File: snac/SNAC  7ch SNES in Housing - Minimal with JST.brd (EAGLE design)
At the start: 63.6 x 64.1 mm, 8 parts, among them U1 PMIC-LDO-XC6206P332MR-G(SOT23), X2 JST-XH-09-PIN-LONG-PAD

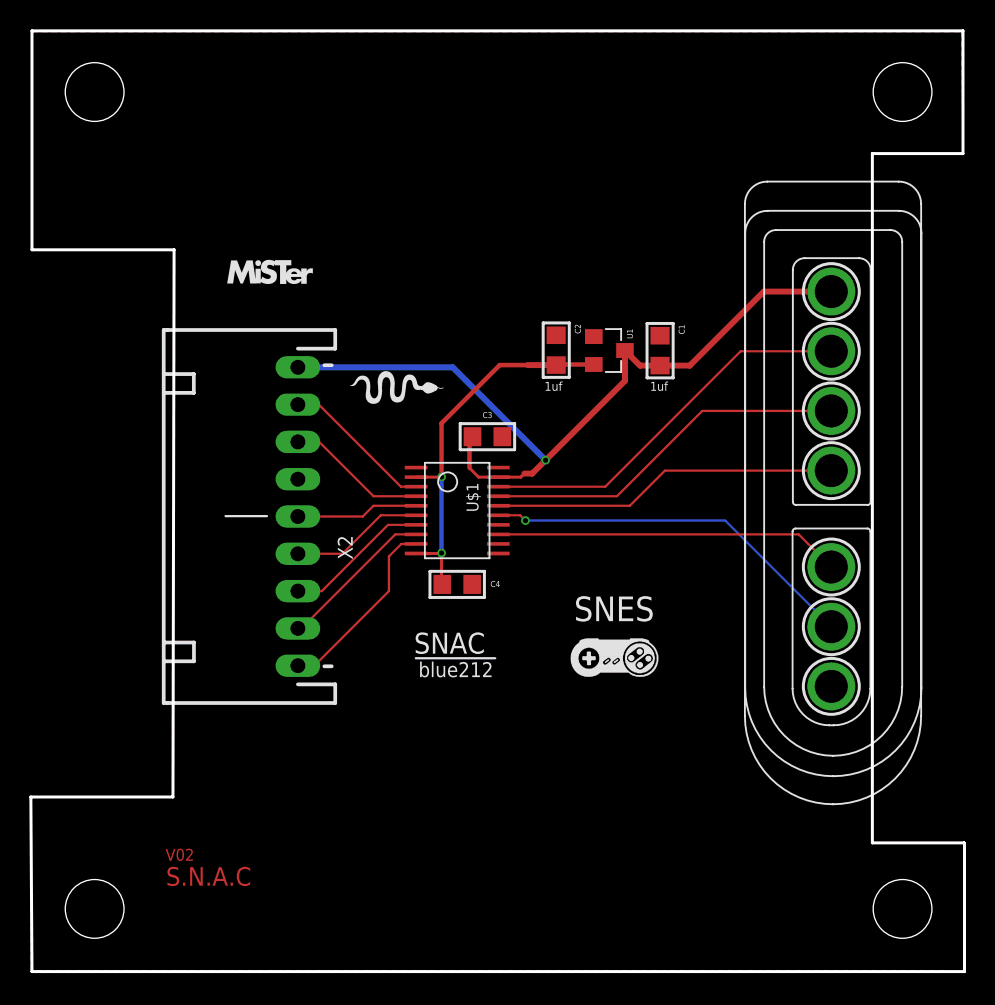
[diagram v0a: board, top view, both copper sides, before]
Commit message: SMS 3D and SNES SNAC JST updates
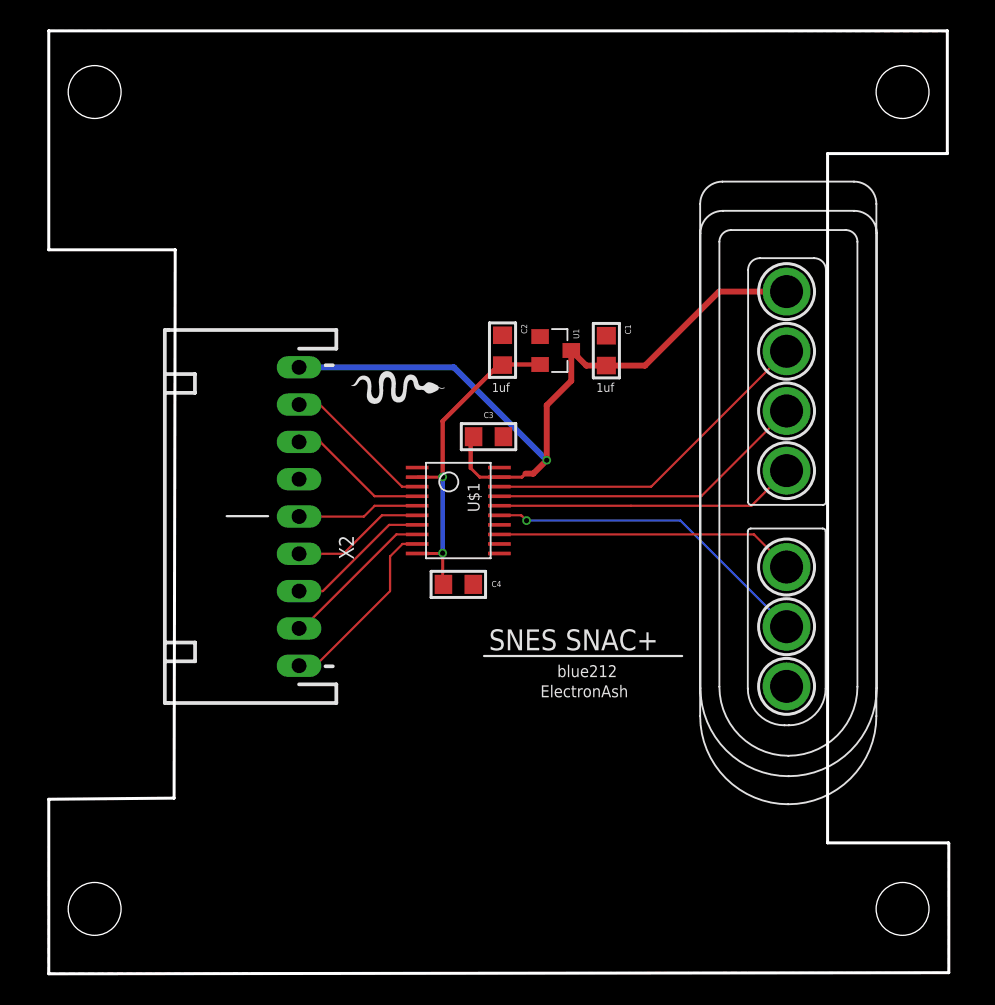
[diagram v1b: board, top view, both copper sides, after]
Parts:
- moved C1 3.66 mm to (51.4, 42.9)
- moved C2 3.66 mm to (44.3, 42.9)
- moved U1 3.66 mm to (47.9, 42.9)
- moved U$3 3.05 mm to (59.6, 46.9)
- moved C3 0.08 mm to (43.4, 37.0)
- moved C4 0.08 mm to (41.3, 27.0)
- moved U$1 0.08 mm to (41.3, 32.0)
- moved X2 0.08 mm to (30.5, 31.6)
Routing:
- net LV: track 26.5 -> 22.9 mm
- net HV4: track 25.1 -> 22.0 mm
- net HV1: track 23.6 -> 20.5 mm
- net HV6: track 23.7 -> 20.5 mm
- net HV5: track 25.8 -> 22.7 mm
- net HV2: track 26.5 -> 23.4 mm
- net HV: track 54.1 -> 53.2 mm
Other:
- board size 63.6 x 64.1 mm -> 61.3 x 64.2 mm
- board text added: "ElectronAsh"
- board text added: "SNES SNAC+"
- board text removed: "S.N.A.C"
- board text removed: "SNAC"
- board text removed: "SNES"
- board text removed: "V02"
